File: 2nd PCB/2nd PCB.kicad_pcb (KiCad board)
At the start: 2 copper layers, 40 x 40 mm, 16 parts, among them J1 Battery, J2 ADC PIN, J3 PWM PIN, J4 DC Moter (Brushes), J5 L298N Module, J6 Sensor/Main PCB, Q1 NMOS, U1 ACS712xLCTR-05B, U2 L7805

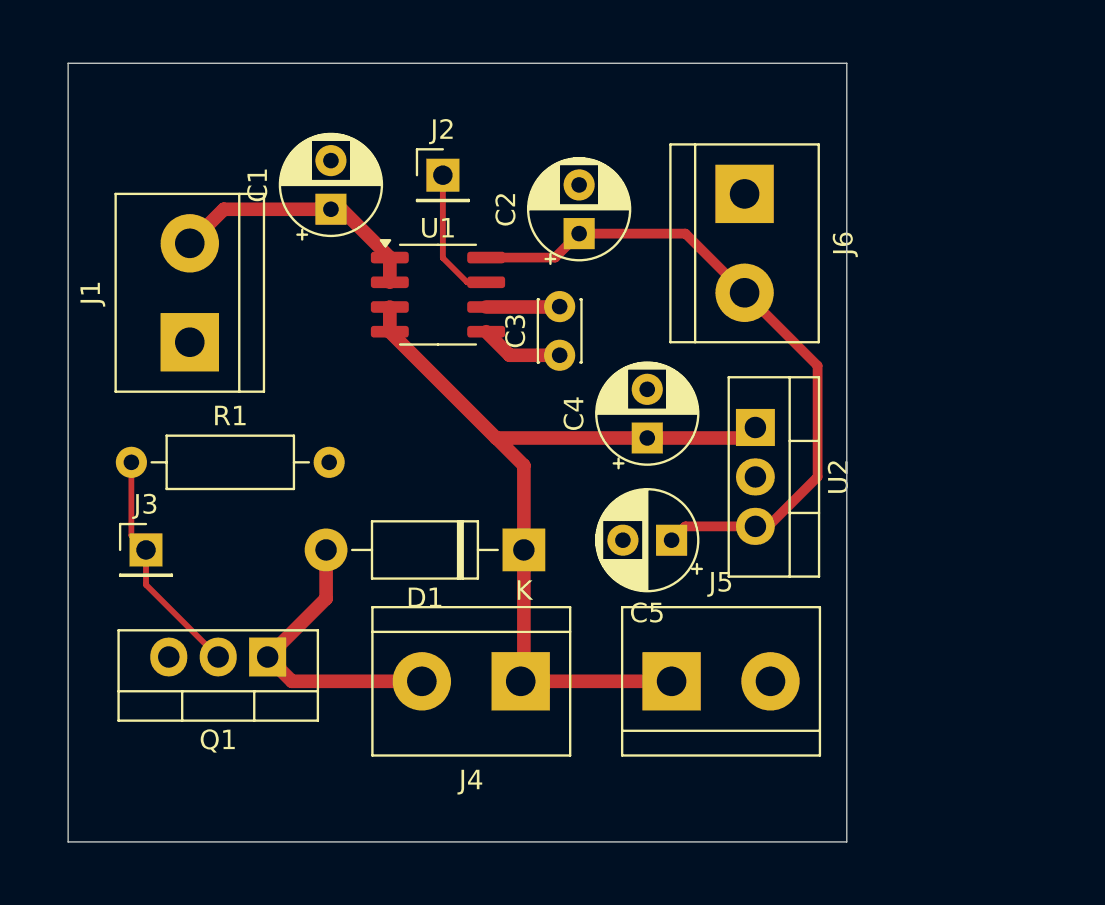
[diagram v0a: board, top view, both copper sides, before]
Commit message: finished the PCB board designs
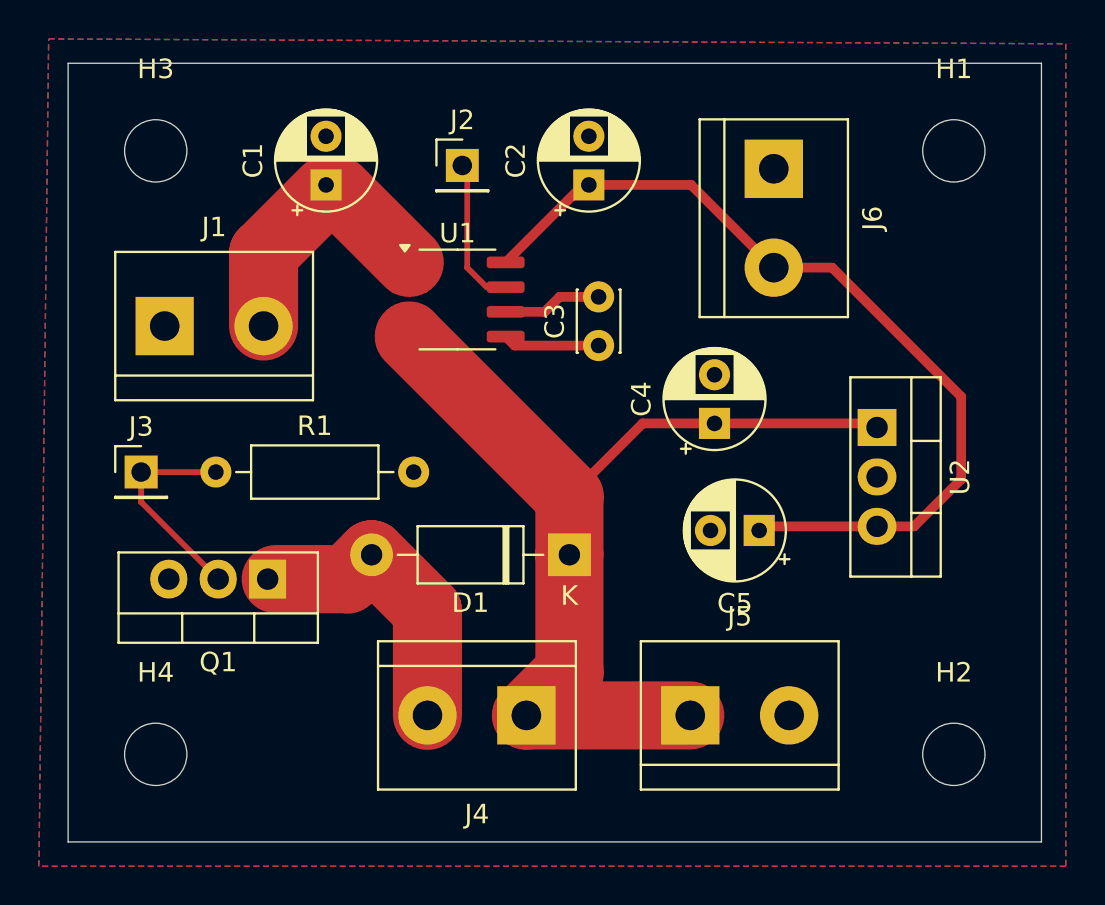
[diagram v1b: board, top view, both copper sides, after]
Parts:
- added H1: MountingHole, MountingHole:MountingHole_3.2mm_M3, F.Cu at (145.8, 82.2)
- added H2: MountingHole, MountingHole:MountingHole_3.2mm_M3, F.Cu at (145.8, 113.2)
- added H3: MountingHole, MountingHole:MountingHole_3.2mm_M3, F.Cu at (104.8, 82.2)
- added H4: MountingHole, MountingHole:MountingHole_3.2mm_M3, F.Cu at (104.8, 113.2)
- moved U2 6.25 mm to (141.8, 96.5)
- moved C5 4.53 mm to (135.8, 101.8)
- moved R1 4.37 mm to (107.8, 98.8)
- moved J3 4.01 mm to (104.0, 98.8)
- moved Q1 4.00 mm to (110.5, 104.2)
- moved C4 3.54 mm to (133.5, 96.2)
- moved C2 2.55 mm to (127.0, 84.0)
- moved D1 2.35 mm to (126.0, 103.0)
- moved C3 2.06 mm to (127.5, 92.2)
- moved J5 2.00 mm to (132.2, 111.2)
- moved J6 1.98 mm to (136.5, 83.2)
- moved J4 1.77 mm to (123.8, 111.2)
- moved J1 1.53 mm to (105.2, 91.2), turned to 0 degrees
- moved C1 1.27 mm to (113.5, 84.0)
- moved J2 1.12 mm to (120.5, 83.0)
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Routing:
- net +5V: track 34.9 -> 45.3 mm
- net Net-(D1-K): track 43.6 -> 49.7 mm
- net Net-(J2-Pin_1): track 6.99 -> 8.45 mm
- net Net-(U1-FILTER): track 3.78 -> 5.09 mm
- net Net-(J3-Pin_1): track 11.9 -> 11.0 mm
- net Net-(J1-Pin_2): track 13.3 -> 14.1 mm
- net GND: track 4.28 -> 4.97 mm
- net Net-(D1-A): track 15.4 -> 14.9 mm
- added copper zone on B.Cu, net GND
- added copper zone on F.Cu, net GND
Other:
- board size 40 x 40 mm -> 50 x 40 mm
